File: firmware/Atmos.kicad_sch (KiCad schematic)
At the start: 72 parts, among them J1 AS3935 breakout, J2 BME280 breakout, J3 USB_C_Receptacle_USB2.0_16P, J4 Micro_SD_Card, J5 Solar power input, J6 Conn_Coaxial, Q1 PMOS_Substrate, Q2 PMOS_Substrate, Q3 PMOS_Substrate, SW2 SW_Push, U1 ESP32-S3-WROOM-1, U10 TPS22918DBVR, U11 MAX17048G_T10, U12 CN3791, U13 SGP40-D-R4, U2 AP2112K-3.3, U3 DS3231M, U4 PMS5003, U5 LTC4412xS6, U7 RFM95W-915S2, U8 USBLC6-2SC6, U9 TPS61023DRLR

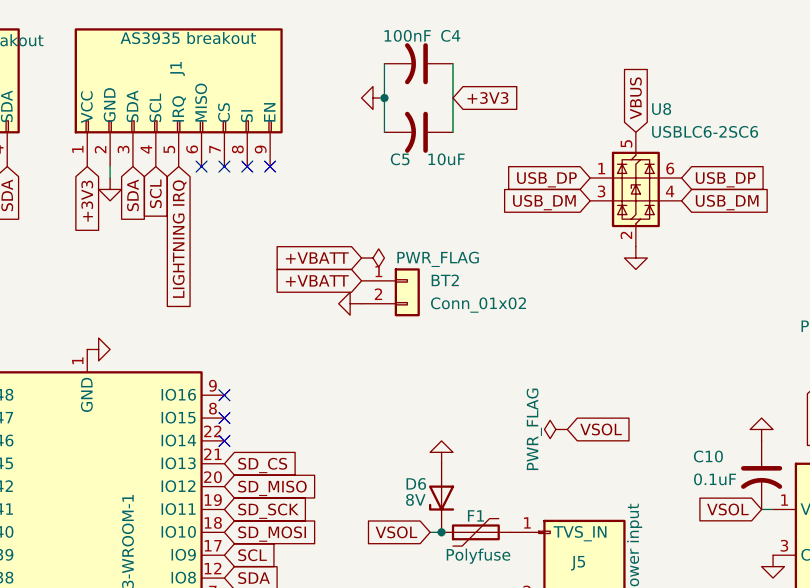
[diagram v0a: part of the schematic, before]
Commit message: updated a few values
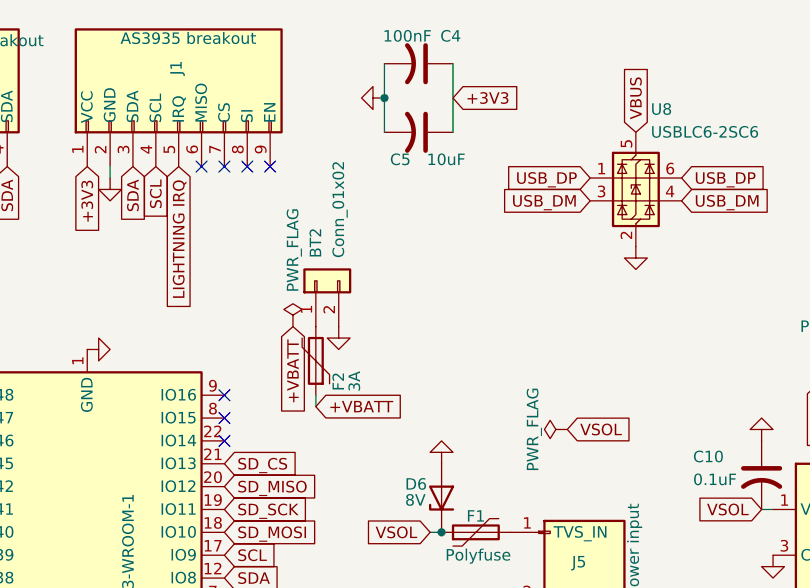
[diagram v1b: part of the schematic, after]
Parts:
- added F2: 3A, symbol Device:Polyfuse
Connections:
- net +VBATT: now also F2.1; no longer BT2.1 (Pin_1)
- new net: BT2.1 (Pin_1), F2.2
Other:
- moved on the sheet: BT2
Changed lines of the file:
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@@
 	(wire
 		(pts
+			(xy 121.92 55.88) (xy 121.92 54.61)
+		)
+		(stroke
+			(width 0)
+			(type default)
+		)
+	)
+	(wire
+		(pts
 			(xy 195.58 78.74) (xy 195.58 81.28)
 		)
@@
 	(global_label "+VBATT"
 		(shape input)
-		(at 127 41.91 180)
+		(at 121.92 55.88 0)
 		(fields_autoplaced yes)
 		(effects
@@
 				(size 1.27 1.27)
 			)
-			(justify right)
+			(justify left)
 		)
 		(property "Intersheetrefs" "${INTERSHEET_REFS}"
-			(at 117.06 41.91 0)
+			(at 131.86 55.88 0)
 			(effects
 				(font
 					(size 1.27 1.27)
 				)
-				(justify right)
+				(justify left)
 				(hide yes)
 			)
@@
 	(global_label "+VBATT"
 		(shape input)
-		(at 127 39.37 180)
+		(at 119.38 46.99 270)
 		(fields_autoplaced yes)
 		(effects
@@
 		)
 		(property "Intersheetrefs" "${INTERSHEET_REFS}"
-			(at 117.06 39.37 0)
+			(at 119.38 56.93 90)
 			(effects
 				(font
@@
 	(symbol
 		(lib_id "power:PWR_FLAG")
-		(at 127 39.37 270)
+		(at 119.38 46.99 0)
 		(unit 1)
 		(exclude_from_sim no)
@@
 		(fields_autoplaced yes)
 		(property "Reference" "#FLG05"
-			(at 128.905 39.37 0)
+			(at 119.38 45.085 0)
 			(effects
 				(font
@@
 		)
 		(property "Value" "PWR_FLAG"
-			(at 130.81 39.3699 90)
+			(at 119.3799 43.18 90)
 			(effects
 				(font
@@
 		)
 		(property "Footprint" ""
-			(at 127 39.37 0)
+			(at 119.38 46.99 0)
 			(effects
 				(font
@@
 		)
 		(property "Datasheet" "~"
-			(at 127 39.37 0)
+			(at 119.38 46.99 0)
 			(effects
 				(font
@@
 		)
 		(property "Description" "Special symbol for telling ERC where power comes from"
-			(at 127 39.37 0)
+			(at 119.38 46.99 0)
 			(effects
 				(font
@@
 	(symbol
 		(lib_id "Connector_Generic:Conn_01x02")
-		(at 132.08 41.91 0)
+		(at 121.92 41.91 90)
 		(unit 1)
 		(exclude_from_sim no)
@@
 		(fields_autoplaced yes)
 		(property "Reference" "BT2"
-			(at 134.62 41.9099 0)
+			(at 121.9199 39.37 0)
 			(effects
 				(font
@@
 		)
 		(property "Value" "Conn_01x02"
-			(at 134.62 44.4499 0)
+			(at 124.4599 39.37 0)
 			(effects
 				(font
@@
 		)
 		(property "Footprint" ""
-			(at 132.08 41.91 0)
+			(at 121.92 41.91 0)
 			(effects
 				(font
@@
 		)
 		(property "Datasheet" "~"
-			(at 132.08 41.91 0)
+			(at 121.92 41.91 0)
 			(effects
 				(font
@@
 		)
 		(property "Description" "Generic connector, single row, 01x02, script generated (kicad-library-utils/schlib/autogen/connector/)"
-			(at 132.08 41.91 0)
+			(at 121.92 41.91 0)
 			(effects
 				(font
@@
 	)
 	(symbol
+		(lib_id "Device:Polyfuse")
+		(at 121.92 50.8 180)
+		(unit 1)
+		(exclude_from_sim no)
+		(in_bom yes)
+		(on_board yes)
+		(dnp no)
+		(property "Reference" "F2"
+			(at 124.46 53.086 90)
+			(effects
+				(font
+					(size 1.27 1.27)
+				)
+			)
+		)
+		(property "Value" "3A"
+			(at 126.238 53.086 90)
+			(effects
+				(font
+					(size 1.27 1.27)
+				)
+			)
+		)
+		(property "Footprint" ""
+			(at 120.65 45.72 0)
+			(effects
+				(font
+					(size 1.27 1.27)
+				)
+				(justify left)
+				(hide yes)
+			)
+		)
+		(property "Datasheet" "~"
+			(at 121.92 50.8 0)
+			(effects
+				(font
+					(size 1.27 1.27)
+				)
+				(hide yes)
+			)
+		)
+		(property "Description" "Resettable fuse, polymeric positive temperature coefficient"
+			(at 121.92 50.8 0)
+			(effects
+				(font
+					(size 1.27 1.27)
+				)
+				(hide yes)
+			)
+		)
+		(pin "2"
+		)
+		(pin "1"
+		)
+		(instances
+			(project ""
+				(path "/821c823f-0cdf-48e4-87e1-02b442913dca"
+					(reference "F2")
+					(unit 1)
+				)
+			)
+		)
+	)
+	(symbol
 		(lib_id "Simulation_SPICE:PMOS_Substrate")
 		(at 182.88 55.88 90)
@@
 	(symbol
 		(lib_id "power:GND")
-		(at 127 44.45 270)
+		(at 124.46 46.99 0)
 		(unit 1)
 		(exclude_from_sim no)
@@
 		(fields_autoplaced yes)
 		(property "Reference" "#PWR034"
-			(at 120.65 44.45 0)
+			(at 124.46 53.34 0)
 			(effects
 				(font
@@
 		)
 		(property "Value" "GND"
-			(at 123.19 44.4499 90)
+			(at 124.4599 50.8 90)
 			(effects
 				(font
@@
 		)
 		(property "Footprint" ""
-			(at 127 44.45 0)
+			(at 124.46 46.99 0)
 			(effects
 				(font
@@
 		)
 		(property "Datasheet" ""
-			(at 127 44.45 0)
+			(at 124.46 46.99 0)
 			(effects
 				(font
@@
 		)
 		(property "Description" "Power symbol creates a global label with name \"GND\" , ground"
-			(at 127 44.45 0)
+			(at 124.46 46.99 0)
 			(effects
 				(font
